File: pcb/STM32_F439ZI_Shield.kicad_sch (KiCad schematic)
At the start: 19 parts, among them K1 G6S-2, K2 G6S-2, U1 LM2904, U13 R-78E3.3-0.5, U14 R-78E5.0-0.5, U2 MAX3485

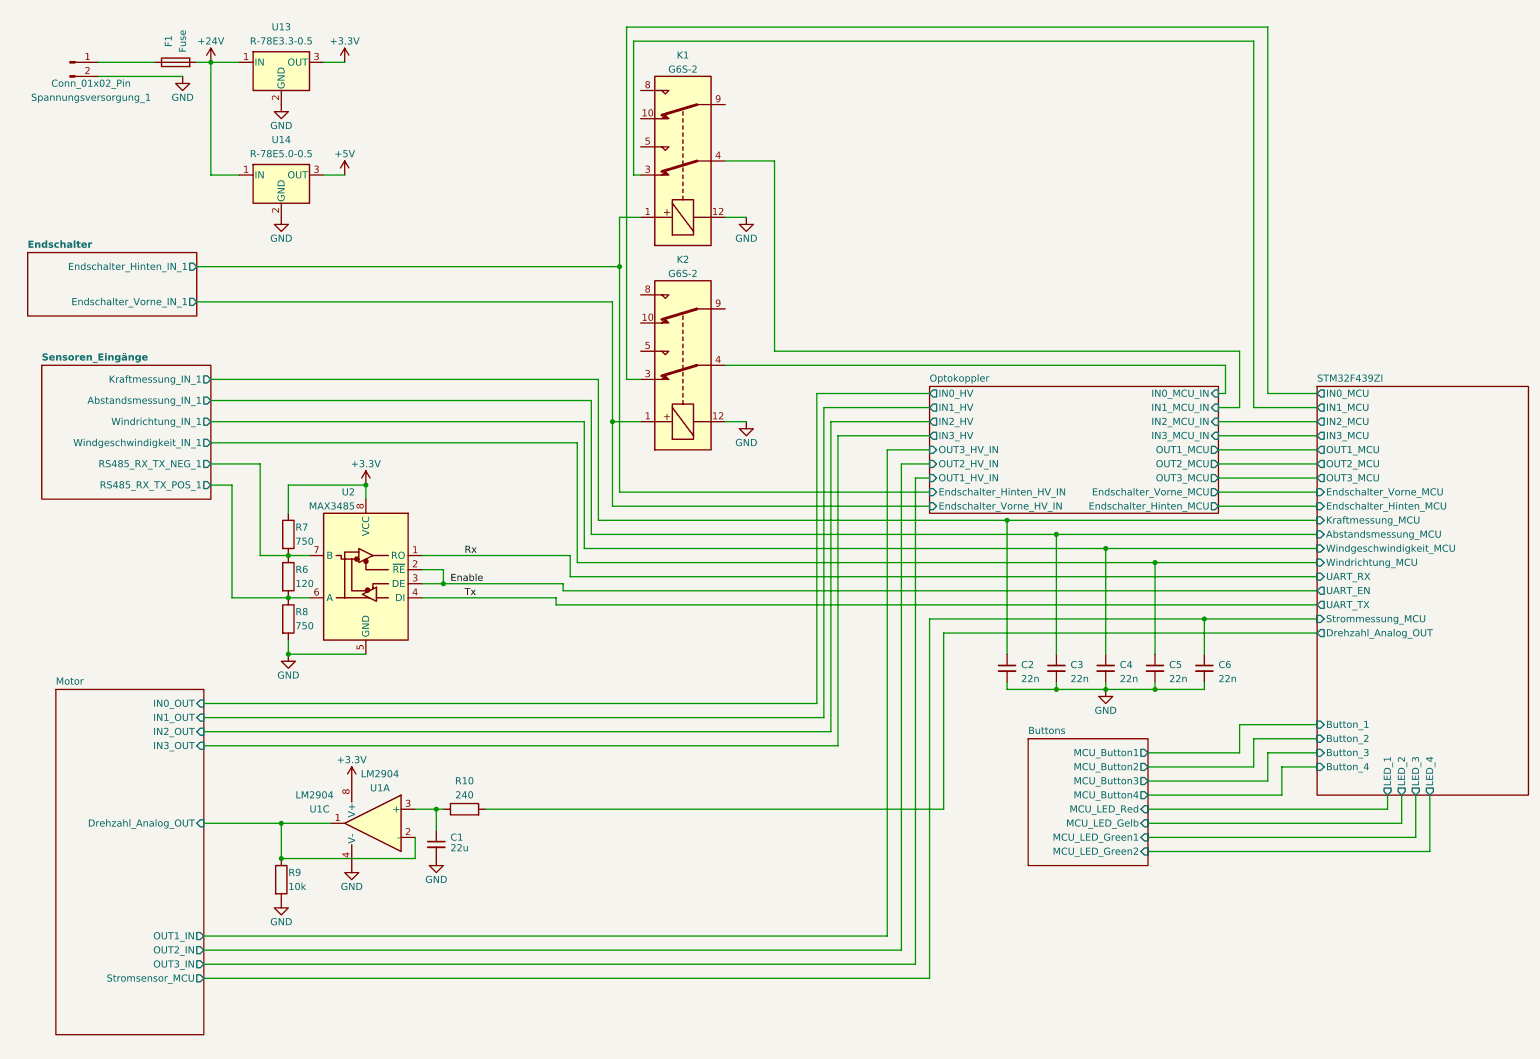
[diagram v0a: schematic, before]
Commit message: updated pcb
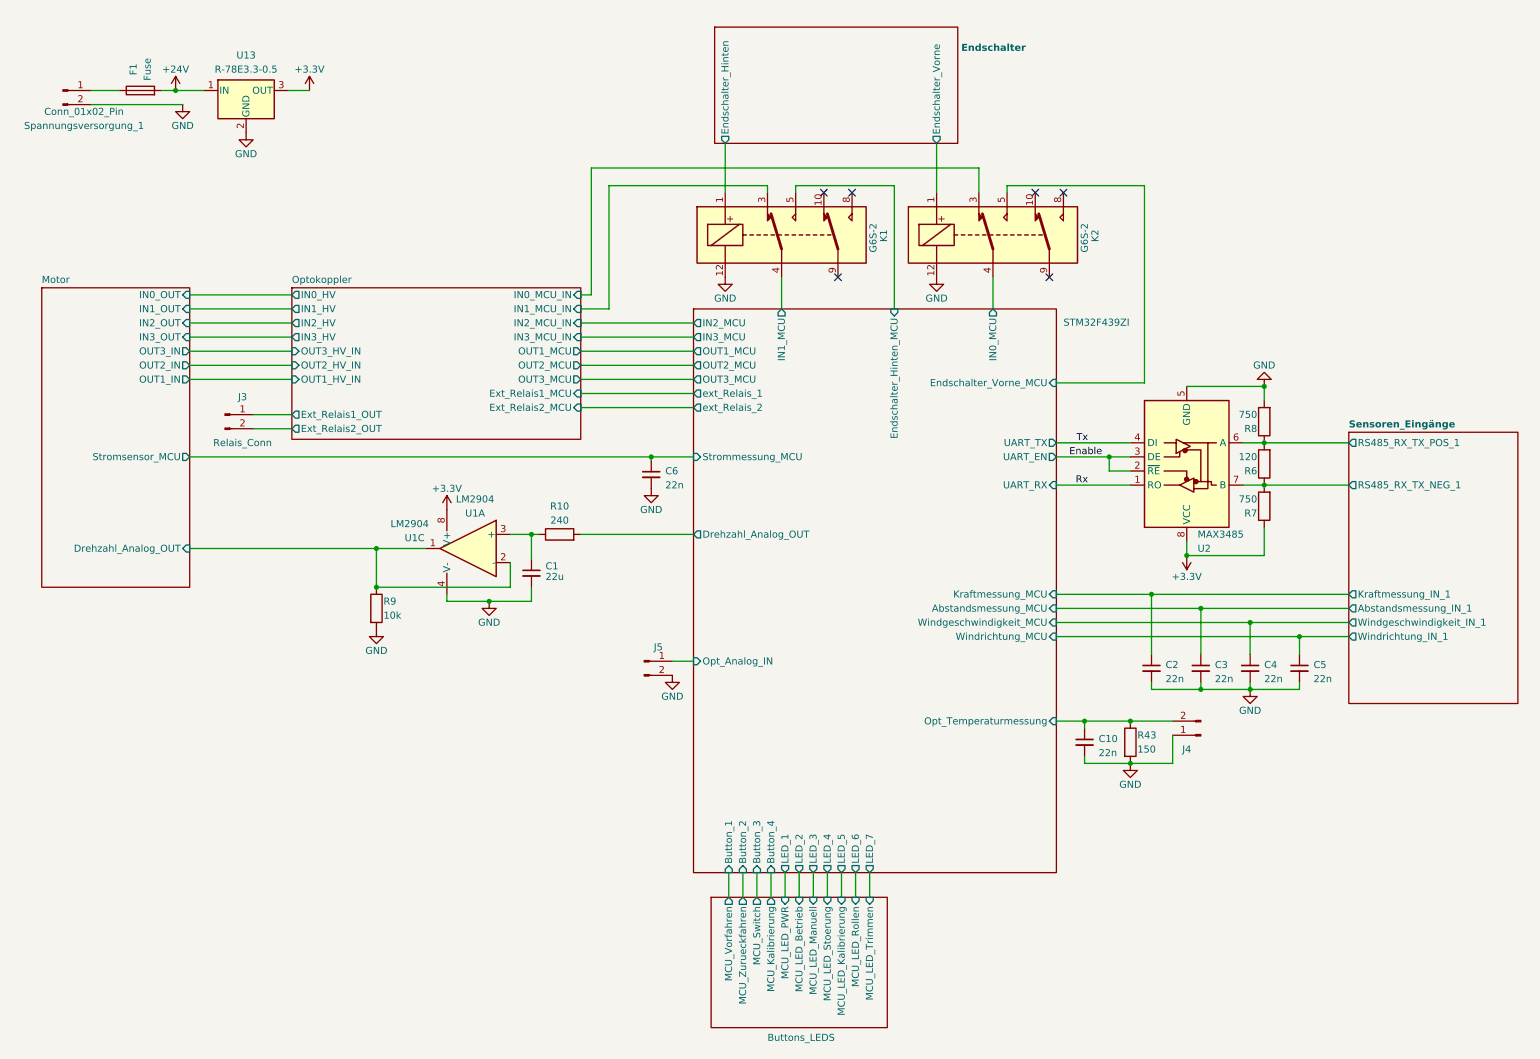
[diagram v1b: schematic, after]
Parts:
- removed U14: R-78E5.0-0.5, Converter_DCDC:Converter_DCDC_RECOM_R-78E-0.5_THT, symbol Regulator_Switching:R-78E5.0-0.5
- added C10: 22n, Capacitor_SMD:C_1206_3216Metric, symbol Device:C_Small
- added J3: Relais_Conn, TerminalBlock_TE-Connectivity:TerminalBlock_TE_282834-2_1x02_P2.54mm_Horizontal, symbol Connector:Conn_01x02_Pin
- added J4, J5: Conn_01x02_Pin, TerminalBlock_TE-Connectivity:TerminalBlock_TE_282834-2_1x02_P2.54mm_Horizontal, symbol Connector:Conn_01x02_Pin
- added R43: 150, Resistor_SMD:R_1206_3216Metric, symbol Device:R
- Spannungsversorgung_1: footprint Connector_Phoenix_MSTB:PhoenixContact_MSTBA_2,5_2-G-5,08_1x02_P5.08mm_Horizontal -> TerminalBlock_TE-Connectivity:TerminalBlock_TE_282834-2_1x02_P2.54mm_Horizontal
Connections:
- net GND: now also C10.2, J4.1 (Pin_1), J5.2 (Pin_2), R43.2
- net Optokoppler/IN0_MCU_IN: now also K2.3; no longer K2.4
- net Optokoppler/IN1_MCU_IN: now also K1.3; no longer K1.4
- net STM32F439ZI/IN0_MCU: now also K2.4; no longer K2.3
- net STM32F439ZI/IN1_MCU: now also K1.4; no longer K1.3
- net STM32F439ZI/Endschalter_Vorne_MCU: now reaches K2.5
- net STM32F439ZI/Endschalter_Hinten_MCU: now reaches K1.5
- net Endschalter/Endschalter_Hinten_IN_1 renamed Endschalter/Endschalter_Hinten
- net Endschalter/Endschalter_Vorne_IN_1 renamed Endschalter/Endschalter_Vorne
- new net Optokoppler/Ext_Relais1_OUT: J3.1 (Pin_1)
- new net Optokoppler/Ext_Relais2_OUT: J3.2 (Pin_2)
- new net STM32F439ZI/Opt_Analog_IN: J5.1 (Pin_1)
- new net STM32F439ZI/Opt_Temperaturmessung: C10.1, J4.2 (Pin_2), R43.1
- no-connect marks 0 -> 6
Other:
- sheet Buttons renamed Buttons_LEDS
- sheet Buttons_LEDS ports: added MCU_Kalibrierung, MCU_LED_Betrieb, MCU_LED_Kalibrierung, MCU_LED_Manuell, MCU_LED_PWR, MCU_LED_Rollen, MCU_LED_Stoerung, MCU_LED_Trimmen, MCU_Switch, MCU_Vorfahren, MCU_Zurueckfahren; removed MCU_Button1, MCU_Button2, MCU_Button3, MCU_Button4, MCU_LED_Gelb, MCU_LED_Green1, MCU_LED_Green2, MCU_LED_Red
- sheet Endschalter ports: added Endschalter_Hinten, Endschalter_Vorne; removed Endschalter_Hinten_IN_1, Endschalter_Vorne_IN_1
- sheet Optokoppler ports: added Ext_Relais1_MCU, Ext_Relais1_OUT, Ext_Relais2_MCU, Ext_Relais2_OUT; removed Endschalter_Hinten_HV_IN, Endschalter_Hinten_MCU, Endschalter_Vorne_HV_IN, Endschalter_Vorne_MCU
- sheet STM32F439ZI ports: added LED_5, LED_6, LED_7, Opt_Analog_IN, Opt_Temperaturmessung, ext_Relais_1, ext_Relais_2; removed none
- moved on the sheet: C1, C2, C3, C4, C5, C6, F1, K1, K2, R10, R6, R7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
